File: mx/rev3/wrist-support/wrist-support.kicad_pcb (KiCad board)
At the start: 2 copper layers, 88 x 65 mm, 4 parts

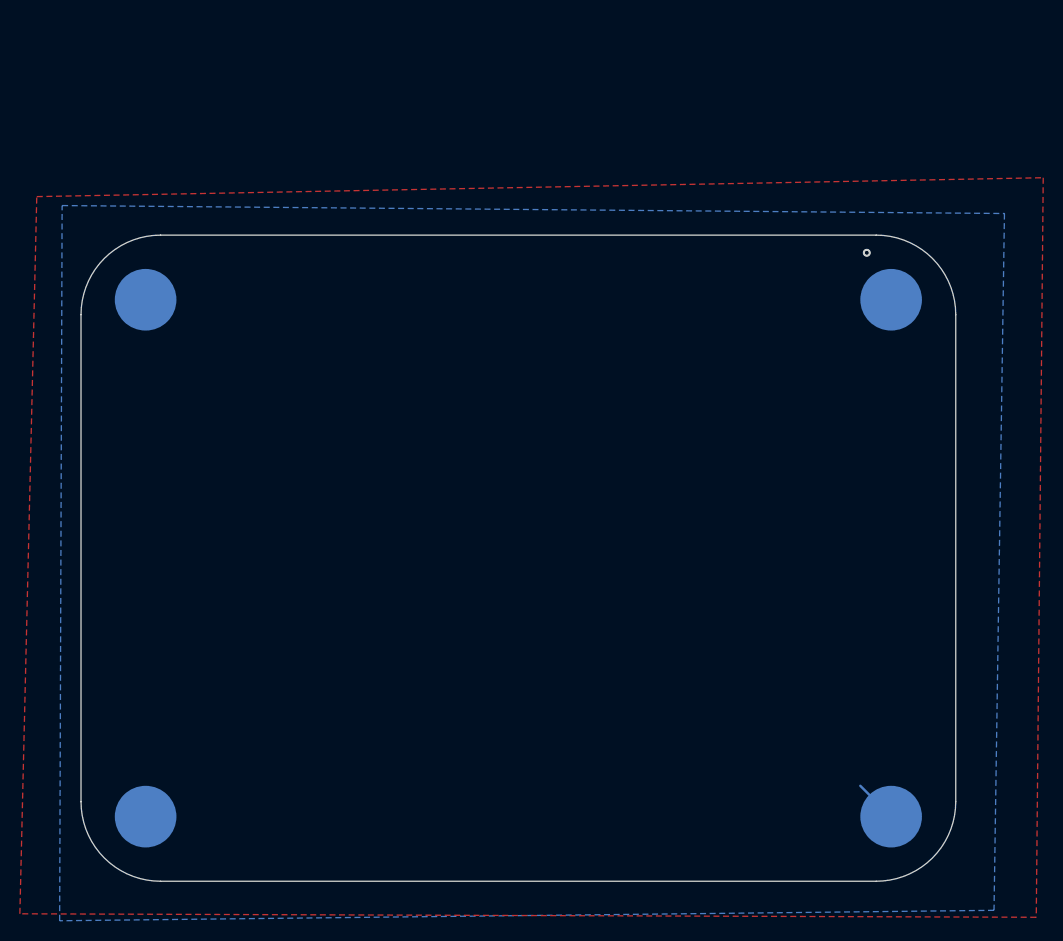
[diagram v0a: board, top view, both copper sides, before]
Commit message: M giri-kicad-lib/switches.kicad_sym  M giri-kicad-lib/switches_lib.pretty/C_0603_1608Metric.kicad_mod  M giri-kicad-lib/switches_lib.pretty/Gateron_1u.kicad_mod  M giri-kicad-lib/switches_lib.pretty/Gateron_Sw_1u.kicad_mod  M giri-kicad-lib/switches_lib.pretty/PGA2040_SMT_WITH_SLOT.kicad_mod  M giri-kicad-lib/switches_lib.pretty/Pad_Only_SMTSO_M2.kicad_mod  M giri-kicad-lib/switches_lib.pretty/SW_B3U-3000P.kicad_mod  D giri-kicad-lib/switches_lib.pretty/WristExtension.kicad_mod A  mx/rev3/Wrist-Plate2/Wrist-Plate2.kicad_pcb A  mx/rev3/Wrist-Plate2/Wrist-Plate2.kicad_prl A  mx/rev3/Wrist-Plate2/Wrist-Plate2.kicad_pro A  mx/rev3/Wrist-Plate2/Wrist-Plate2.kicad_sch A  mx/rev3/Wrist-Plate2/fp-lib-table M  mx/rev3/border.py R  mx/rev3/pcb/LED-Driver.kicad_sch -> mx/rev3/pcb-rev1/pcb/LED-Driver.kicad_sch R  mx/rev3/pcb/fp-lib-table -> mx/rev3/pcb-rev1/pcb/fp-lib-table R  mx/rev3/pcb/pcb-b.jpg -> mx/rev3/pcb-rev1/pcb/pcb-b.jpg R  mx/rev3/pcb/pcb.jpg -> mx/rev3/pcb-rev1/pcb/pcb.jpg R  mx/rev3/pcb/pcb.kicad_pcb -> mx/rev3/pcb-rev1/pcb/pcb.kicad_pcb A  mx/rev3/pcb-rev1/pcb/pcb.kicad_prl R  mx/rev3/pcb/pcb.kicad_pro -> mx/rev3/pcb-rev1/pcb/pcb.kicad_pro R  mx/rev3/pcb/pcb.kicad_sch -> mx/rev3/pcb-rev1/pcb/pcb.kicad_sch R  mx/rev3/pcb/sym-lib-table -> mx/rev3/pcb-rev1/pcb/sym-lib-table A  mx/rev3/pcb-rev2/pcb/LED-Driver.kicad_sch A  mx/rev3/pcb-rev2/pcb/fp-lib-table A  mx/rev3/pcb-rev2/pcb/pcb-b.jpg A  mx/rev3/pcb-rev2/pcb/pcb.jpg A  mx/rev3/pcb-rev2/pcb/pcb.kicad_pcb R  mx/rev3/pcb/pcb.kicad_prl -> mx/rev3/pcb-rev2/pcb/pcb.kicad_prl A  mx/rev3/pcb-rev2/pcb/pcb.kicad_pro A  mx/rev3/pcb-rev2/pcb/pcb.kicad_sch A  mx/rev3/pcb-rev2/pcb/sym-lib-table D  mx/rev3/pcb/.gitignore M  mx/rev3/place.py A  mx/rev3/switch-plate-wide/fp-lib-table A  mx/rev3/switch-plate-wide/switch-plate-wide.kicad_pcb A  mx/rev3/switch-plate-wide/switch-plate-wide.kicad_prl A  mx/rev3/switch-plate-wide/switch-plate-wide.kicad_pro A  mx/rev3/switch-plate-wide/switch-plate-wide.kicad_sch A  mx/rev3/switch-plat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
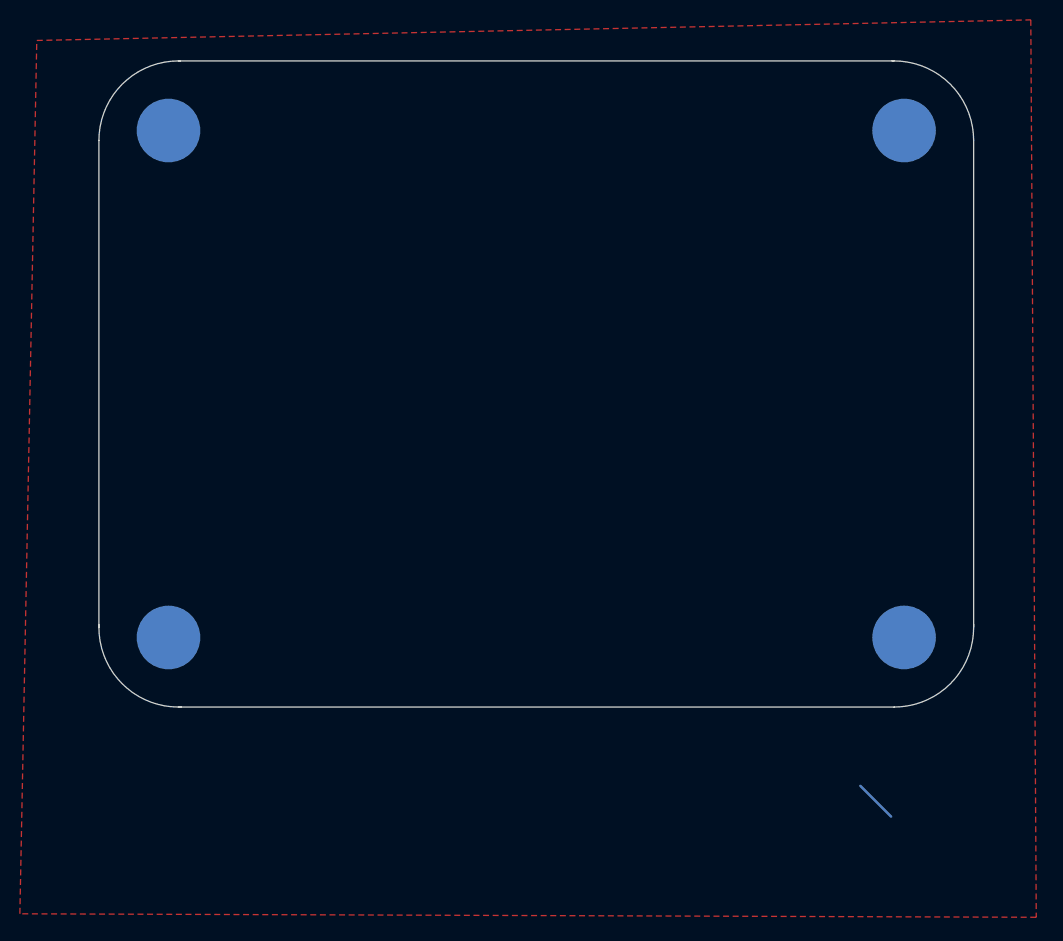
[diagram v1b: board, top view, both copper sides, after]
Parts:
- removed Hs1, Hs2, Hs3, Hs4: TestPoint_Pad, giri:Pad_Only_SMTSO_M2
- added H1: MountingHole_Pad, giri:Pad_Only_SMTSO_M2, F.Cu at (8.80, 27.0)
- added H2: MountingHole_Pad, giri:Pad_Only_SMTSO_M2, F.Cu at (8.80, 78.0)
- added H3: MountingHole_Pad, giri:Pad_Only_SMTSO_M2, F.Cu at (82.8, 78.0)
- added H4: MountingHole_Pad, giri:Pad_Only_SMTSO_M2, F.Cu at (82.8, 27.0)
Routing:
- net GND: vias 1 -> 0
- removed copper zone on B.Cu, net GND
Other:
- outline, holes or cut-outs redrawn
